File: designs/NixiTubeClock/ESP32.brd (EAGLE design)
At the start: 43 x 54 mm, 19 parts, among them IC6 ESP32-WROVER-B

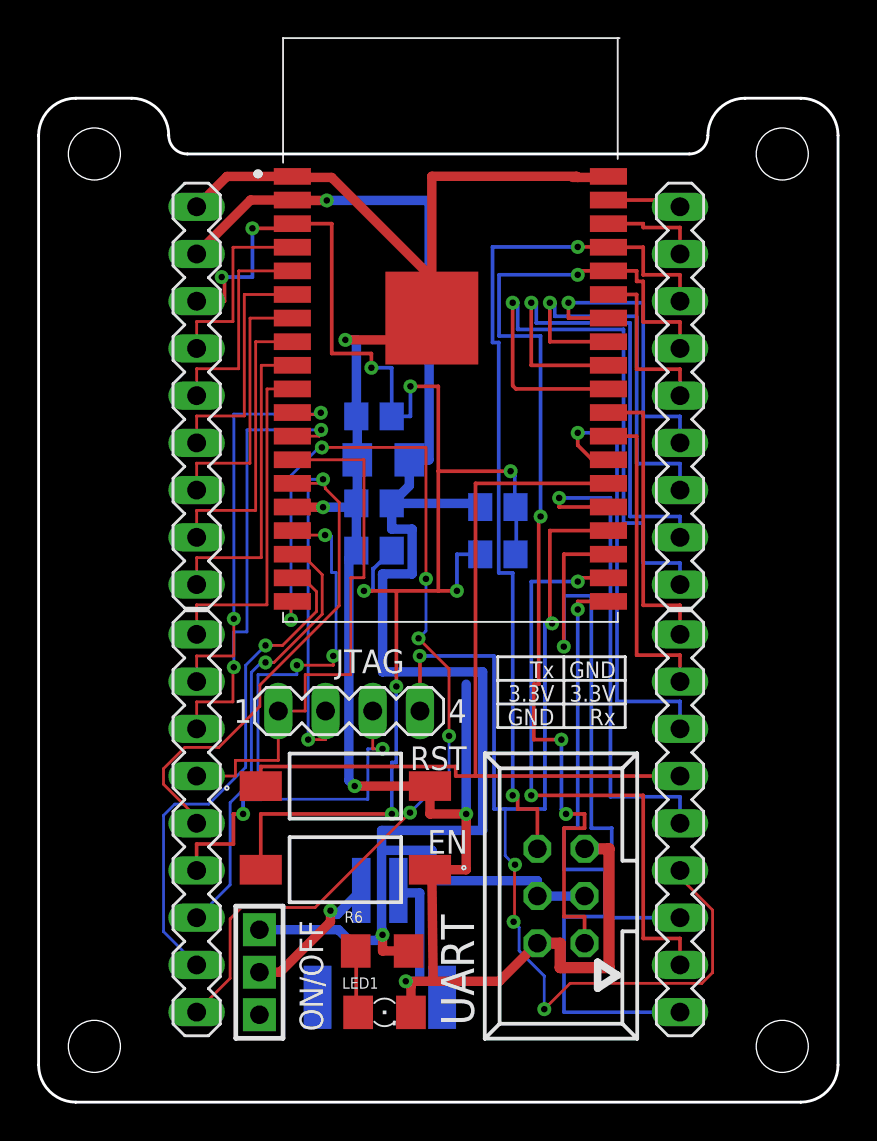
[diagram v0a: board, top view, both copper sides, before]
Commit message: pushed to fusion
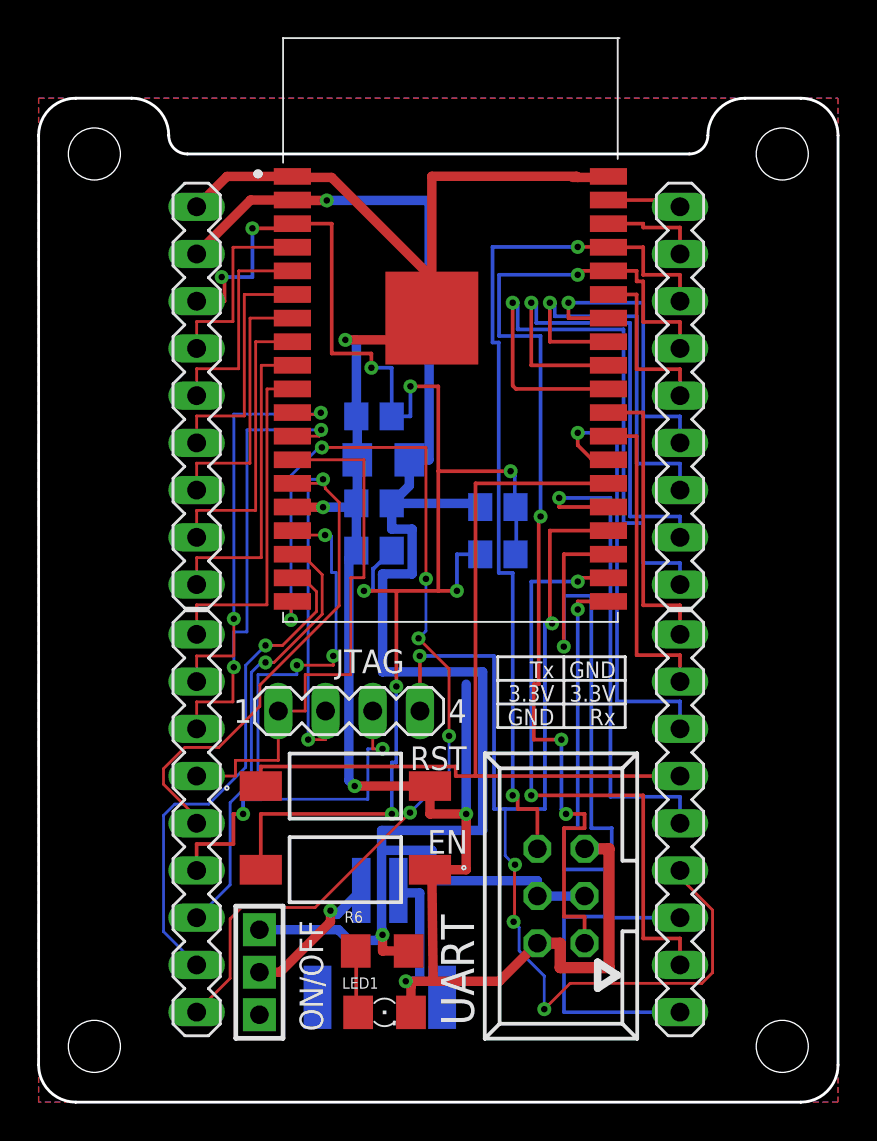
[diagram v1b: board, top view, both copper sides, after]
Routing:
- added copper zone on layer 1, net GND
- added copper zone on layer 16, net GND
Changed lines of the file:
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@@
 <?xml version="1.0" encoding="utf-8"?>
 <!DOCTYPE eagle SYSTEM "eagle.dtd">
-<eagle version="9.4.2">
+<eagle version="9.5.1">
 <drawing>
 <settings>
@@
 </layers>
 <board>
+<fusionsync huburn="a.cGVyc29uYWw6dWUyYTNmMDU1" projecturn="a.cGVyc29uYWw6dWUyYTNmMDU1IzIwMTgxMjEwMTY0OTQ5MjI2" f3durn="urn:adsk.wipprod:dm.lineage:m4VszXO8RDeAbnUYYUwrcQ" pcbguid="13ce3a2b-8468-4712-b890-285fbb146dd9" lastpulledtime="" lastsyncedchangeguid="e74c5fc7-7a09-ba2e-6caf-915c2b94b0bf"/>
 <plain>
 <text x="26.046" y="20.702" size="0.889" layer="25" rot="R180">GND</text>
@@
 <wire x1="12.092" y1="33.887" x2="12.142" y2="33.837" width="0.508" layer="16"/>
 <wire x1="12.142" y1="33.837" x2="12.142" y2="31.547" width="0.508" layer="16"/>
-<wire x1="16.15" y1="38" x2="16.15" y2="39.172" width="0" layer="19" extent="1-1"/>
-<wire x1="16.15" y1="41.35" x2="16.15" y2="39.172" width="0" layer="19" extent="1-1"/>
+<polygon width="0.1524" layer="1">
+<vertex x="-5" y="51"/>
+<vertex x="38" y="51"/>
+<vertex x="38" y="-3"/>
+<vertex x="-5" y="-3"/>
+</polygon>
+<polygon width="0.1524" layer="16">
+<vertex x="-5" y="51"/>
+<vertex x="38" y="51"/>
+<vertex x="38" y="-3"/>
+<vertex x="-5" y="-3"/>
+</polygon>
 </signal>
 <signal name="3.3V">
@@
 </note>
 <note version="8.3" severity="warning">
+Since Version 8.3, EAGLE supports Fusion synchronisation.
+This feature will not be available in this version and saving
+the document will break the link to the Fusion PCB feature.
+</note>
+<note version="8.3" severity="warning">
